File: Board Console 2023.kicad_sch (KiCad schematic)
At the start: 33 parts, among them J1 Raspberry PI, J2 Composite OUT, J3 L1/L2, J5 USB_B_Micro, J6 Display, J7 USB_A, J8 R1/R2, SW10 A, SW11 X, SW12 Down, SW13 Left, SW14 Up, SW15 Right, SW17 SuperDX, SW3 Vol -, SW4 SuperSX, SW5 Select, SW6 Vol +, SW7 Start, SW8 B, SW9 Y

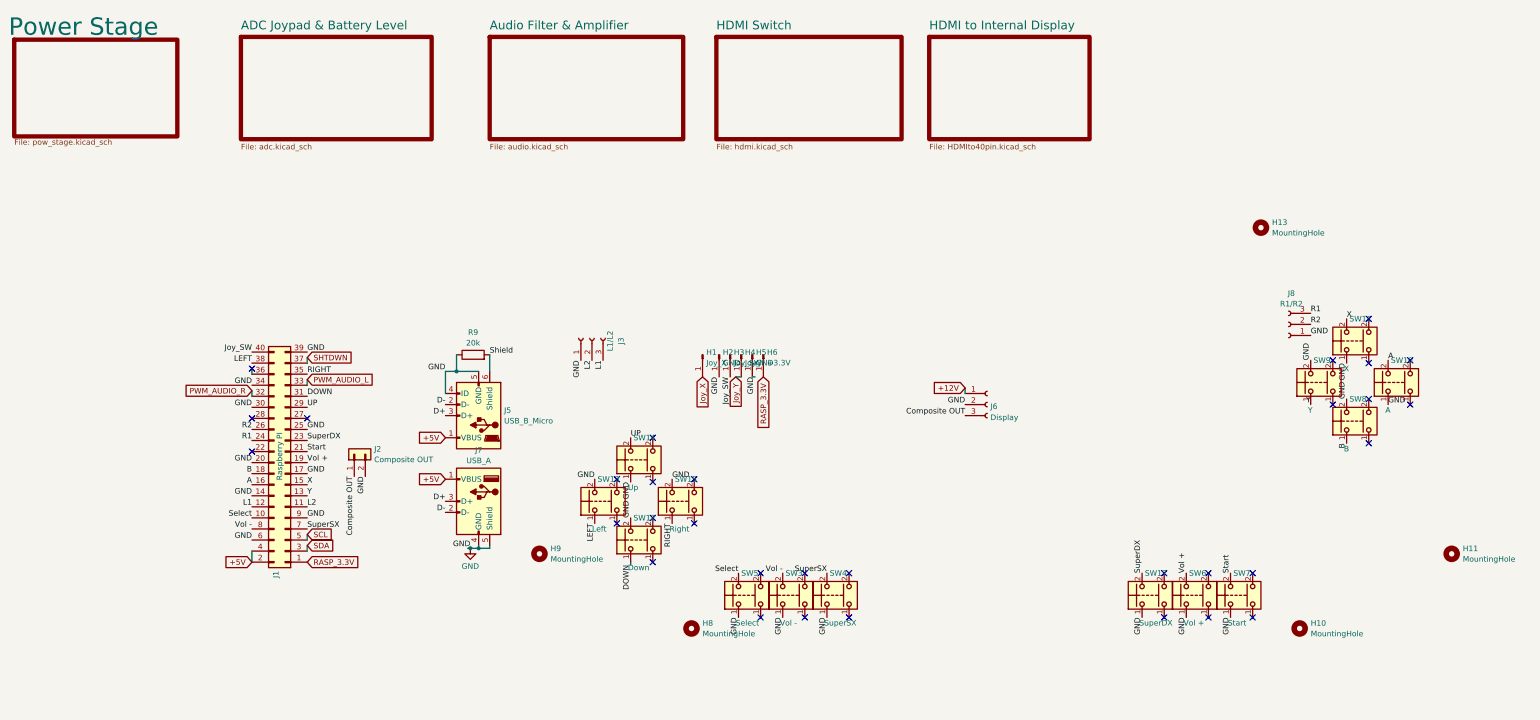
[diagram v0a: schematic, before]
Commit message: update layout pcb & zip tesi
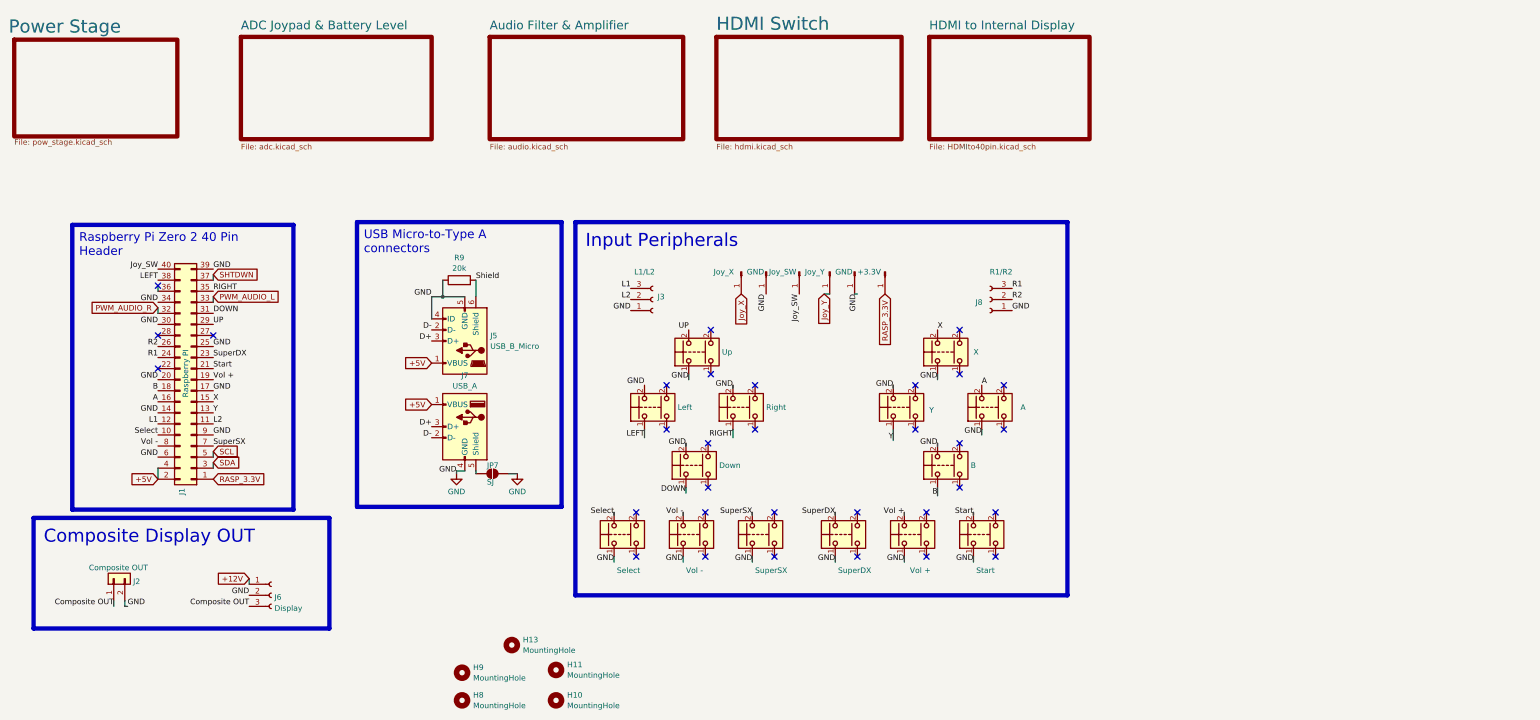
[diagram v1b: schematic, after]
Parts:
- added JP7: SJ, Jumper:SolderJumper-2_P1.3mm_Open_Pad1.0x1.5mm, symbol Jumper:SolderJumper_2_Open
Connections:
- net GND: now also JP7.1 (A); no longer J7.5 (Shield)
- new net: J7.5 (Shield), JP7.2 (B)
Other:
- moved on the sheet: H10, H11, H13, H8, H9, J1, J2, J3, J5, J6, J7, J8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
